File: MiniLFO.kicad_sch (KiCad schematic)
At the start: 19 parts, among them J1 IDC_2x05, U1 TL074

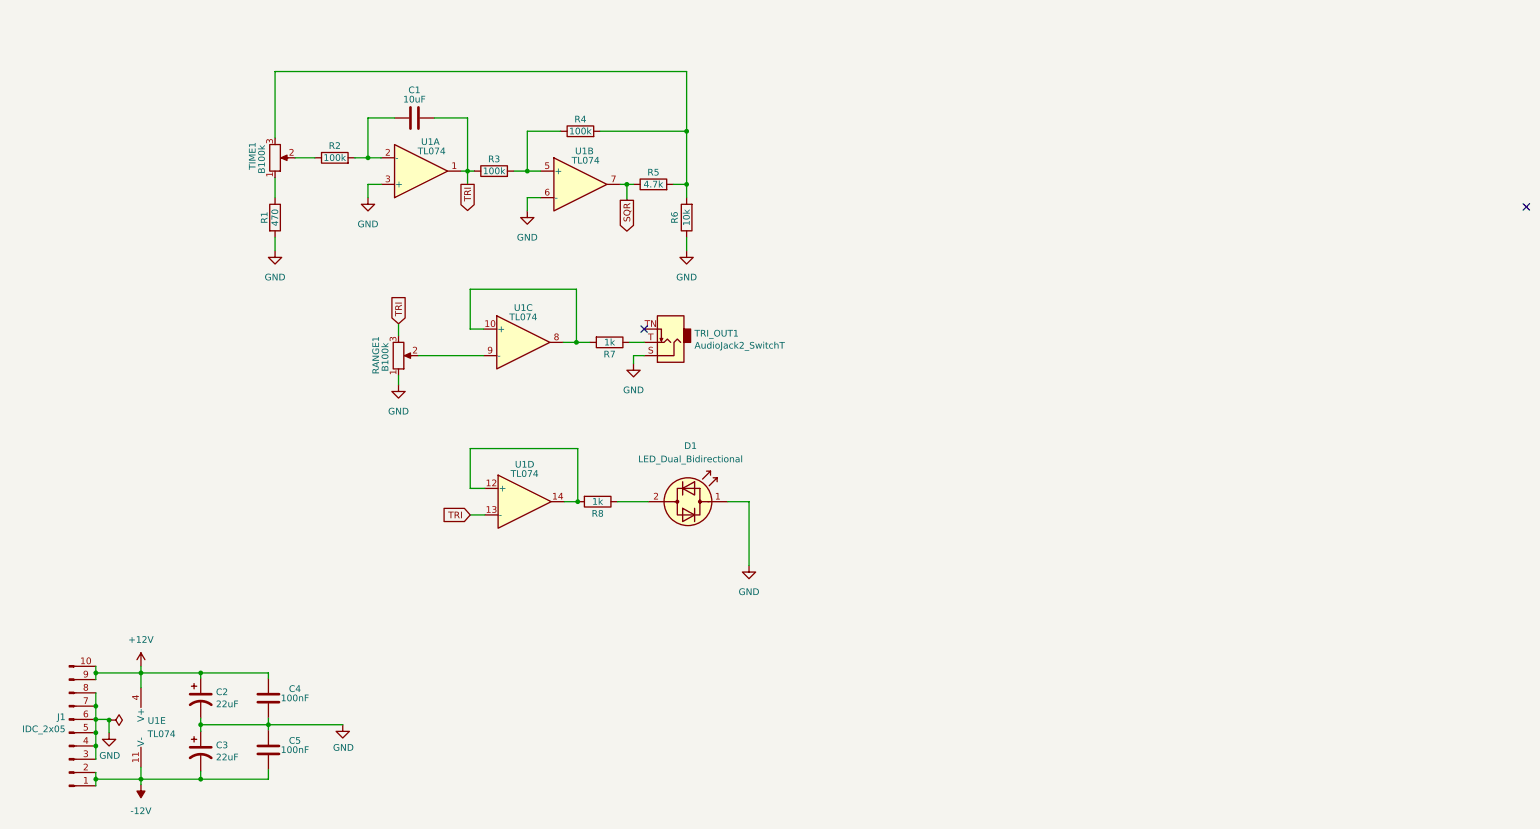
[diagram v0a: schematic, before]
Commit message: hello git
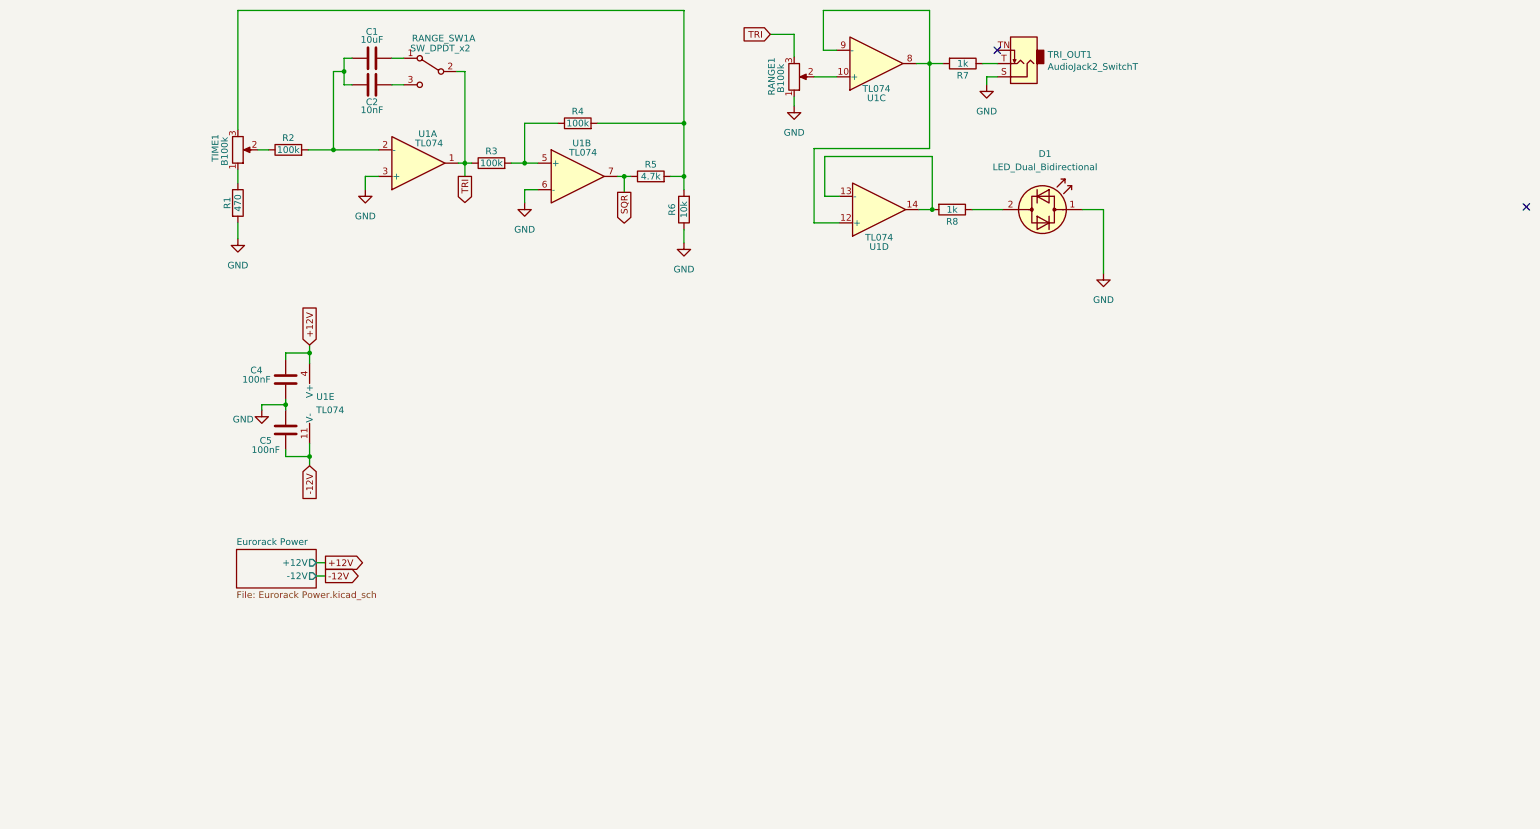
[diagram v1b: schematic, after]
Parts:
- removed C2, C3: 22uF, Capacitor_SMD:C_0805_2012Metric_Pad1.18x1.45mm_HandSolder, symbol MiniDelay-rescue:CP1-Device
- removed J1: IDC_2x05, Connector_IDC:IDC-Header_2x05_P2.54mm_Vertical, symbol Connector:Conn_01x10_Male
- added C2: 10nF, Capacitor_SMD:C_0805_2012Metric_Pad1.18x1.45mm_HandSolder, symbol Device:C
- added RANGE_SW1: SW_DPDT_x2, benjiaomodular:ToggleSwitch_MTS-202_DPDT, symbol Switch:SW_DPDT_x2
- C1: footprint Capacitor_THT:CP_Radial_D6.3mm_P2.50mm -> Capacitor_SMD:C_0805_2012Metric_Pad1.18x1.45mm_HandSolder
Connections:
- net TRI: now also RANGE_SW1.2 (B); no longer C1.2, U1.13 (-)
- net at R8.2, U1.14: now also U1.13 (-); no longer U1.12 (+)
- net at U1.9 (-): now also R7.2, U1.12 (+), U1.8; no longer RANGE1.2
- net at C1.1, R2.2, U1.2 (-): now also C2.1
- new net: RANGE1.2, U1.10 (+)
- new net: C1.2, RANGE_SW1.1 (A)
- new net: C2.2, RANGE_SW1.3 (C)
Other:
- added sheet Eurorack Power (Eurorack Power.kicad_sch)
- moved on the sheet: C1, C4, C5, D1, R1, R2, R3, R4, R5, R6, R7, R8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
